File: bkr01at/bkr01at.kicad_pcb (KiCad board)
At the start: 2 copper layers, 44 parts, among them J1 Conn_02x03_Odd_Even, J2 Conn_01x02, SW1 SW_Push, SW2 SW_Push, SW3 SW_Push, U1 nRF52832-QFAB, U2 LIS2DH, Y1 32.768kHz, Y2 32MHz

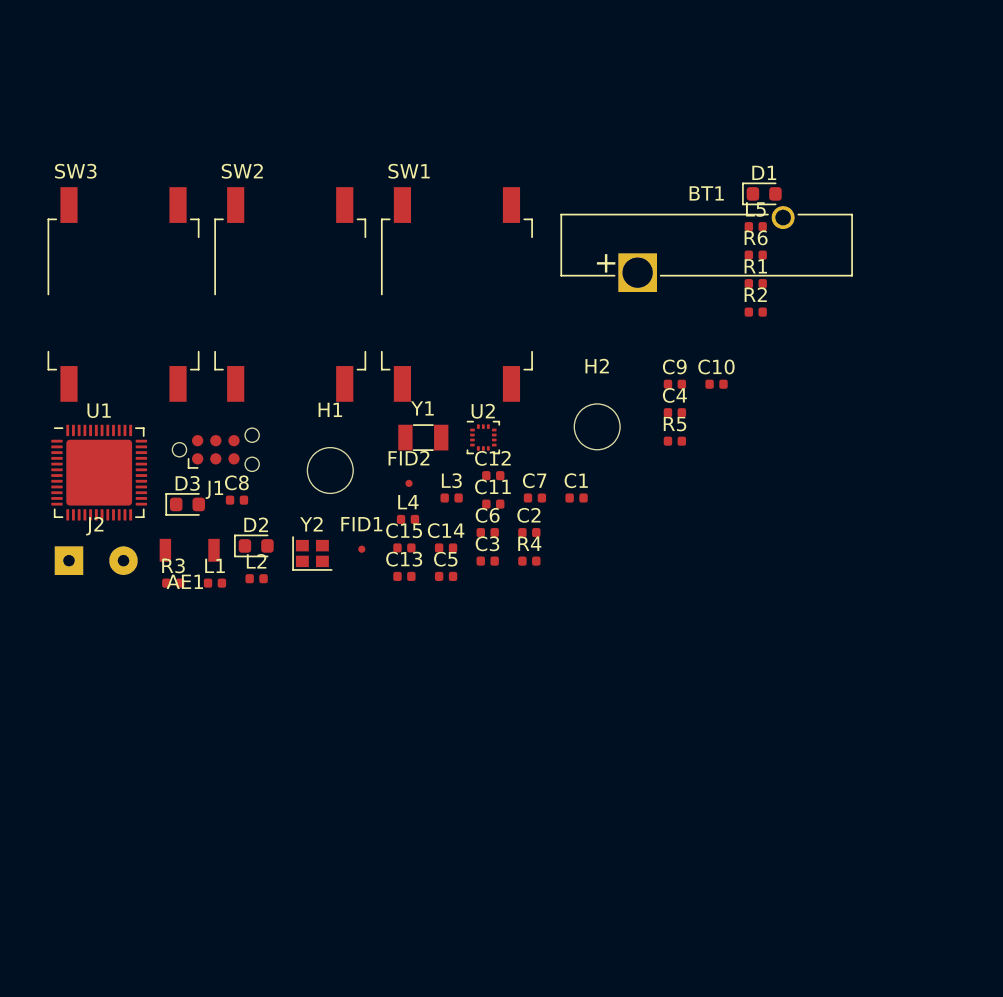
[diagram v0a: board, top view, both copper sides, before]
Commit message: Finalizando PCB.
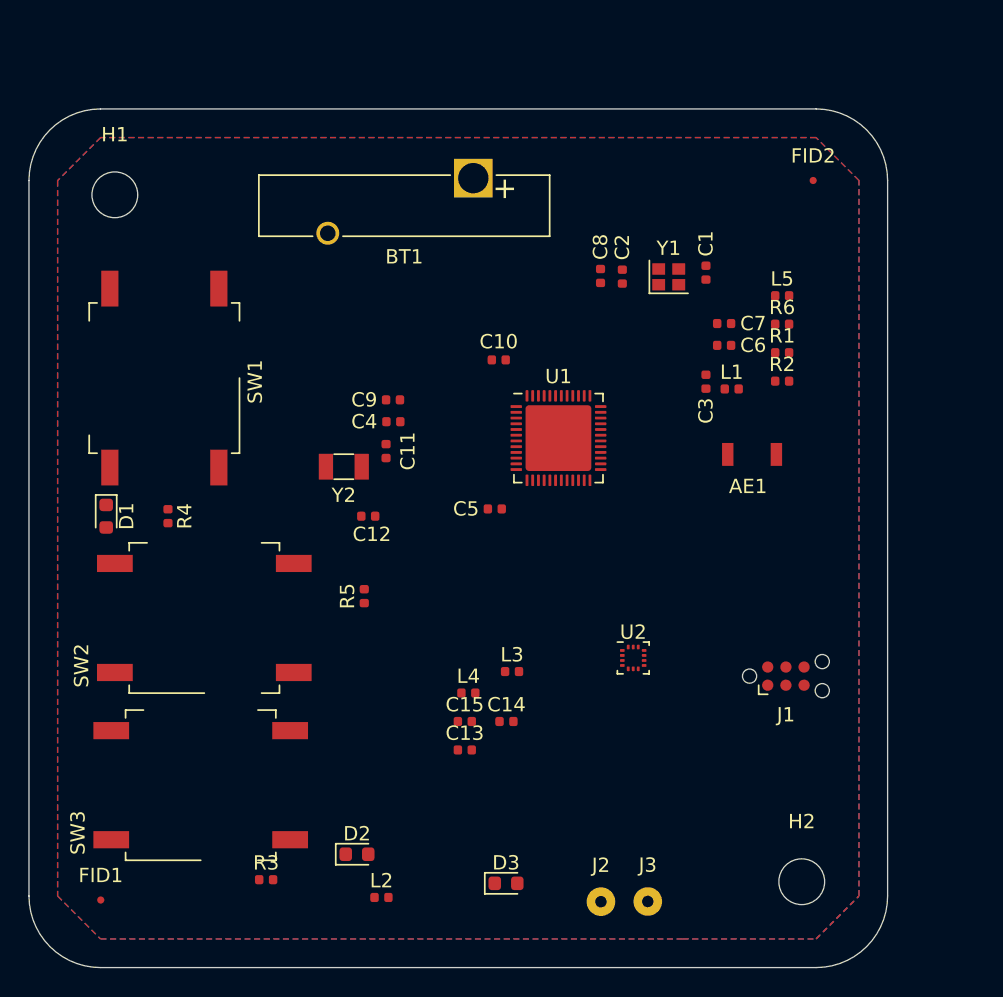
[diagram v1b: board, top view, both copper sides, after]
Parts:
- added J3: Conn_01x01, Connector_Wire:SolderWirePad_1x01_Drill0.8mm, F.Cu at (158.2, 135.4)
- C10: value 1pF -> 1uF
- J2: value Conn_01x02 -> Conn_01x01; footprint Connector_Wire:SolderWirePad_1x02_P3.81mm_Drill0.8mm -> Connector_Wire:SolderWirePad_1x01_Drill0.8mm
- moved D1 51.2 mm to (120.4, 108.5), turned to 270 degrees
- moved J2 44.2 mm to (155.0, 135.4)
- moved J1 42.9 mm to (167.9, 119.6)
- moved AE1 39.9 mm to (165.5, 104.1)
- moved L1 38.6 mm to (164.1, 99.6)
- moved FID2 35.3 mm to (169.8, 85.0)
- moved H2 34.9 mm to (169.0, 134.0)
- moved SW3 34.7 mm to (127.0, 127.3), turned to 90 degrees
- moved D3 34.6 mm to (148.3, 134.1)
- moved U1 32.2 mm to (152.0, 103.0)
- moved Y1 31.5 mm to (159.7, 91.7)
- moved FID1 30.6 mm to (120.0, 135.3)
- moved C8 29.8 mm to (154.9, 91.7), turned to 90 degrees
- moved R4 25.4 mm to (124.7, 108.5), turned to 270 degrees
- moved H1 24.5 mm to (121.0, 86.0)
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- renumbered Y2 to Y1, Y1 to Y2
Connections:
- J2 pad 1: Net-(J2-Pad1) -> J2
- U1 pad 14: Net-(J2-Pad2) -> J2
- U1 pad 15: Net-(J2-Pad1) -> J3
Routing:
- added copper zone on B.Cu, net GND
- added copper zone on F.Cu, net VDD
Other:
- board outline added: 60 x 60 mm

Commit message: PCB e Esquemático finalizados.
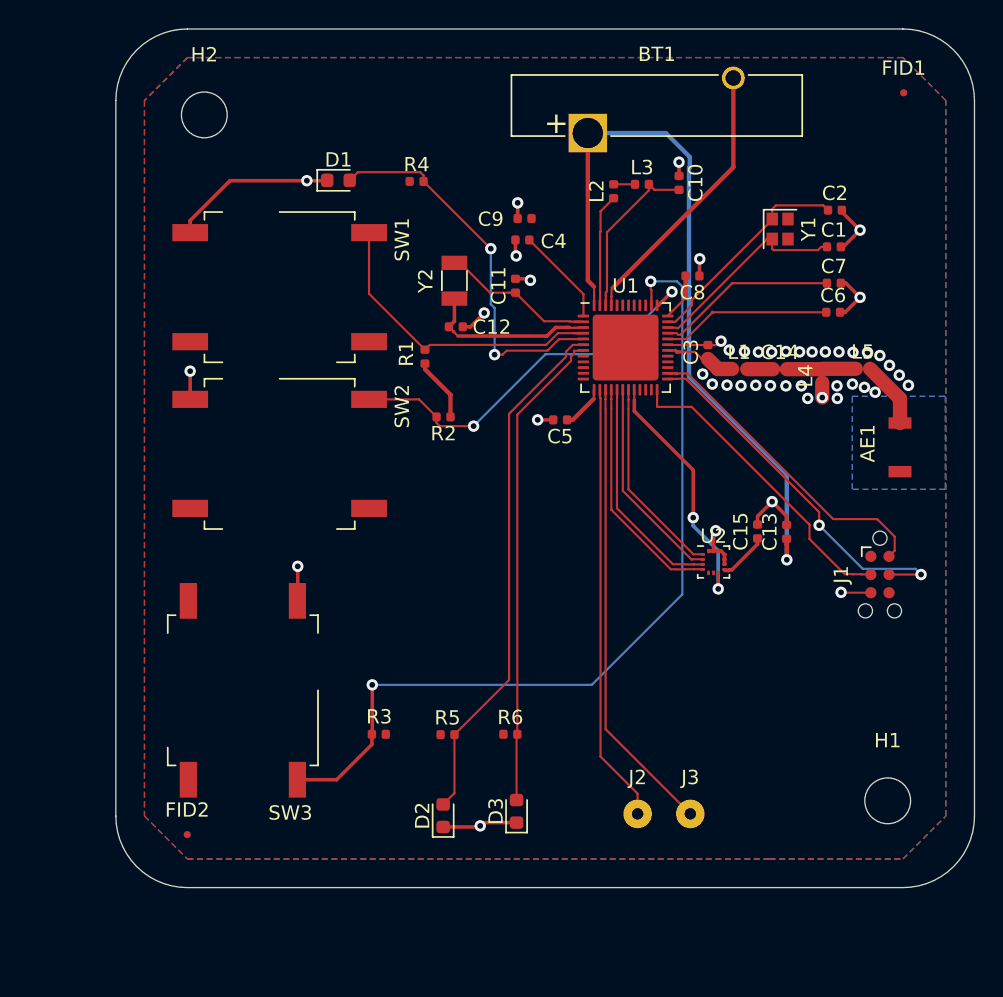
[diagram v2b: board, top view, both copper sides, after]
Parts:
- moved FID1 79.6 mm to (176.1, 78.9)
- moved H1 68.6 mm to (175.0, 128.3)
- moved H2 67.9 mm to (127.3, 80.4)
- moved FID2 63.3 mm to (126.1, 130.7)
- moved L2 52.0 mm to (155.9, 85.8), turned to 90 degrees
- moved L3 35.2 mm to (157.8, 85.3)
- moved R6 34.4 mm to (148.6, 123.7)
- moved L4 33.2 mm to (170.4, 98.7), turned to 90 degrees
- moved C14 31.2 mm to (167.5, 98.2)
- moved R4 29.1 mm to (142.1, 85.1), turned to 0 degrees
- moved D1 28.5 mm to (136.6, 85.0), turned to 0 degrees
- moved C13 27.2 mm to (167.9, 109.6), turned to 90 degrees
- moved R1 25.0 mm to (142.7, 97.3), turned to 90 degrees
- moved C15 24.4 mm to (165.9, 109.5), turned to 90 degrees
- moved R2 23.8 mm to (144.0, 101.5), turned to 180 degrees
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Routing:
- net GND: track 0.00 -> 70.8 mm, vias 0 -> 47
- net VDD: track 0.00 -> 66.8 mm, vias 0 -> 1
- net ButtonF2: track 0.00 -> 60.3 mm, vias 0 -> 2
- net LedT: track 0.00 -> 36.6 mm
- net LedV: track 0.00 -> 33.7 mm
- net J3: track 0.00 -> 32.1 mm
- net J2: track 0.00 -> 30.8 mm
- net ButtonF1: track 0.00 -> 27.6 mm, vias 0 -> 2
- net LedON: track 0.00 -> 26.7 mm, vias 0 -> 2
- net SWDCLK: track 0.00 -> 26.2 mm, vias 0 -> 2
- net SWDIO: track 0.00 -> 22.3 mm
- net RST: track 0.00 -> 21.7 mm
- net ButtonRST: track 0.00 -> 21.7 mm
- net Vdd_IO: track 0.00 -> 17.5 mm, vias 0 -> 2
- net SPI-CS: track 0.00 -> 16.5 mm
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- added copper zone on B.Cu, net VDD
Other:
- net class Default: trace_width 0.25 -> 0.15
- rule solder_mask_min_width: 0.25 -> 0.127
- rule trace_min: 0.2 -> 0.15
